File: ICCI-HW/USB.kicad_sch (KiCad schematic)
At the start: 9 parts

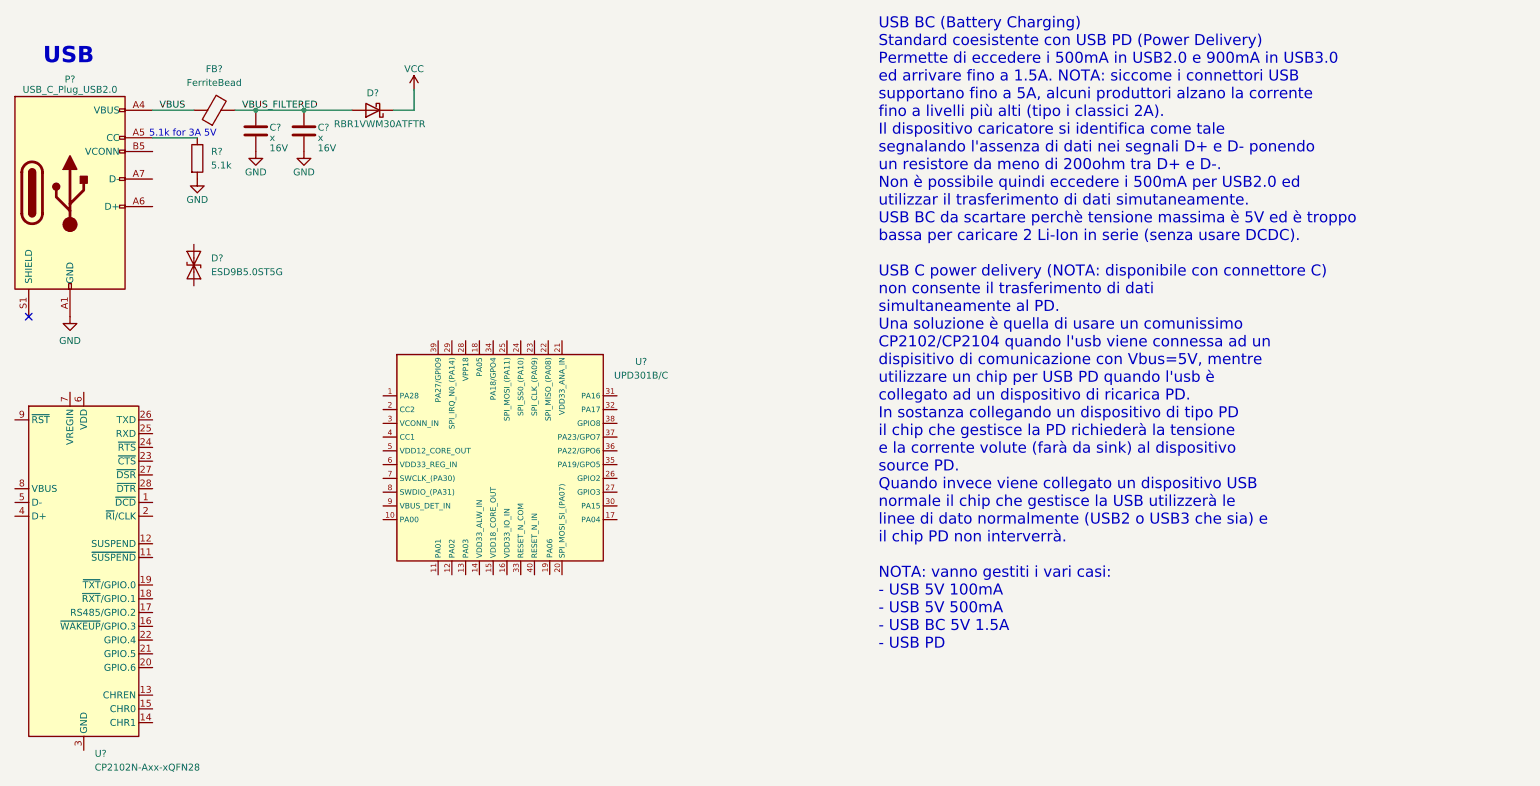
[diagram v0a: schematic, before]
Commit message: updated
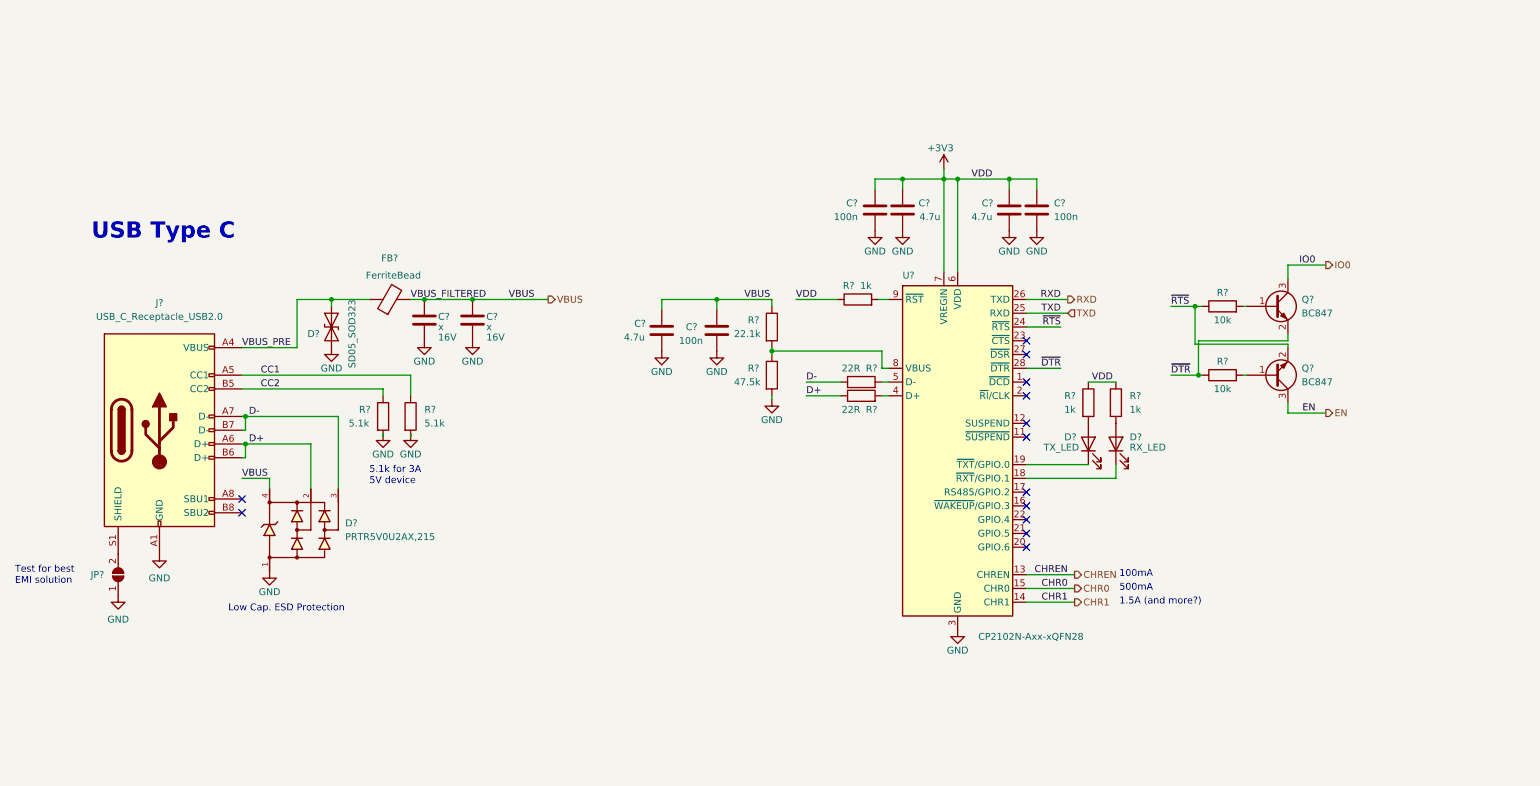
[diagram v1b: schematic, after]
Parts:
- removed D?: RBR1VWM30ATFTR, ppse_2021:Package-PMDE, symbol Device:D_Schottky
- removed D?: ESD9B5.0ST5G, Diode_SMD:D_SOD-923, symbol Diode:ESD9B5.0ST5G
- removed P?: USB_C_Plug_USB2.0, symbol Connector:USB_C_Plug_USB2.0
- removed U?: UPD301B/C, symbol ICCI-LIB:UPD301B/C
- added C? (x3): 100n, symbol Device:C
- added C? (x3): 4.7u, symbol Device:C
- added D?: SD05_SOD323, Diode_SMD:D_SOD-323, symbol Diode:SD05_SOD323
- added D?: TX_LED, symbol Device:LED
- added D?: PRTR5V0U2AX,215, symbol ICCI-LIB:PRTR5V0U2AX,215
- added D?: RX_LED, symbol Device:LED
- added J?: USB_C_Receptacle_USB2.0, Connector_USB:USB_C_Receptacle_Amphenol_12401548E4-2A, symbol Connector:USB_C_Receptacle_USB2.0
- added JP?: SolderJumper_2_Open, symbol Jumper:SolderJumper_2_Open
- added Q? (x2): BC847, Package_TO_SOT_SMD:SOT-23, symbol Transistor_BJT:BC847
- added R? (x2): 10k, symbol Device:R
- added R? (x3): 1k, symbol Device:R
- added R?: 22.1k, symbol Device:R
- added R? (x2): 22R, symbol Device:R
- added R?: 47.5k, symbol Device:R
- added R?: 5.1k, symbol Device:R
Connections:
- net VBUS_FILTERED is gone; now on net VBUS: C?.1, C?.1, FB?.2
- net GND: now also U?.29 (GND), U?.3 (GND), C?.2, C?.2, C?.2, C?.2, C?.2, C?.2, D?.1, D?.1 (A1), J?.A1 (GND), J?.A12 (GND), J?.B1 (GND), J?.B12 (GND), JP?.1 (A), R?.2, R?.2
- net VBUS: now also C?.1, C?.1, D?.4, R?.1; no longer FB?.1
- net CC1: now reaches R?.1
- net CC1: now also J?.A5 (CC1)
- net CHREN: now reaches U?.13 (CHREN)
- net CHR1: now reaches U?.14 (CHR1)
- net CHR0: now reaches U?.15 (CHR0)
- net at U?.18 (~{RXT}/GPIO.1): now also D?.1 (K)
- net at U?.19 (~{TXT}/GPIO.0): now also D?.1 (K)
- net ~{RTS}: now reaches U?.24 (~{RTS})
- net ~{RTS}: now also Q?.2 (E), R?.1
- net TXD: now reaches U?.25 (RXD)
- net RXD: now reaches U?.26 (TXD)
- net ~{DTR}: now reaches U?.28 (~{DTR})
- net ~{DTR}: now also Q?.2 (E), R?.1
- net at U?.4 (D+): now also R?.2
- net at U?.5 (D-): now also R?.2
- net +3V3: now reaches U?.6 (VDD)
- net +3V3: now also U?.7 (VREGIN), C?.1, C?.1, C?.1, C?.1, R?.1, R?.1, R?.1
- net at U?.8 (VBUS): now also R?.1, R?.2
- net at U?.9 (~{RST}): now also R?.2
- new net: Q?.1 (B), R?.2 (x2)
- new net: J?.S1 (SHIELD), JP?.2 (B)
- new net: D?.2 (A), R?.2 (x2)
- new net CC2: J?.B5 (CC2), R?.1
- new net D+: D?.2, J?.A6 (D+), J?.B6 (D+), R?.1
- new net D-: D?.3, J?.A7 (D-), J?.B7 (D-), R?.1
- new net EN: Q?.3 (C)
- new net IO0: Q?.3 (C)
- new net VBUS_PRE: D?.2 (A2), FB?.1, J?.A4 (VBUS), J?.A9 (VBUS), J?.B4 (VBUS), J?.B9 (VBUS)
- no-connect marks 1 -> 13
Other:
- note added: "1.5A (and more?)"
- note added: "100mA"
- note added: "5.1k for 3A 5V device"
- note added: "500mA"
- note added: "Low Cap. ESD Protection"
- note added: "Test for best EMI solution"
- note added: "USB Type C"
- note removed: "5.1k for 3A 5V"
- note removed: "USB"
- note removed: "USB BC (Battery Charging) Standard coesistente con USB PD (Power Delivery) Permette di eccedere i 500mA in USB2.0 e 900mA in USB3.0 ed arrivare fino a 1.5A. NOTA: siccome i connettori USB supportano fino a 5A, alcuni produttori alzano la corrente fino a livelli più alti (tipo i classici 2A). Il dispositivo caricatore si identifica come tale segnalando l'assenza di dati nei segnali D+ e D- ponendo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"
- moved on the sheet: C?, FB?, R?, U?
